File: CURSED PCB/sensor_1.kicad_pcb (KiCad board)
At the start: 4 copper layers, 40 x 40 mm, 68 parts, among them J1 Programming Header, J2 Micro_SD_Card, J3 2 Wire Block for laser, J4 2 Wire Block for PZT, J5 G125-MH104M4-04AD000P, U1 MIC94090YC6, U10 MCP2562, U11 TPS61046YFF, U12 AD5761BRUZ, U2 INA180, U3 STM32G431KBT6, U4 SPX3819M5-L-3-3, U5 MCP1754S-3302xCB, U6 OPA323, U7 MCP3562-E_ST, U8 LTC2066, Y1 24MHz crystal

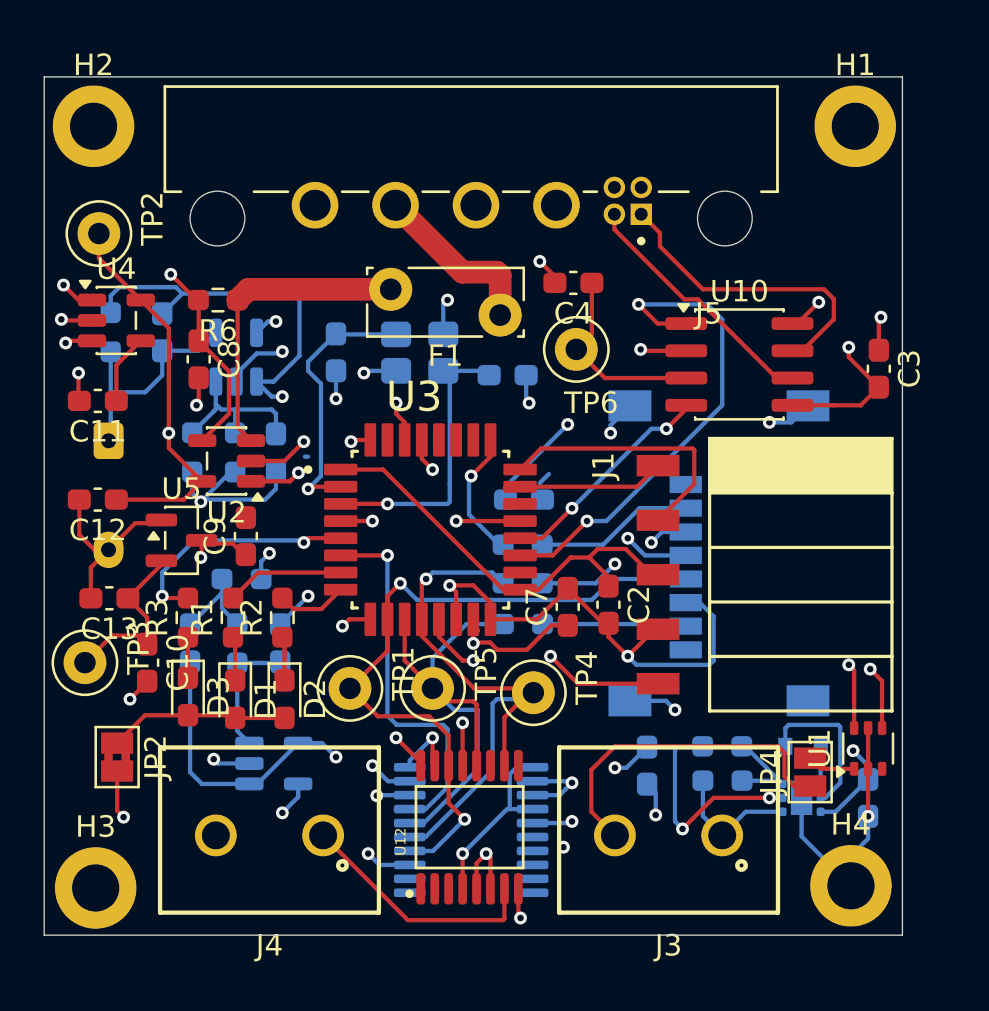
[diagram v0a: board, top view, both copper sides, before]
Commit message: redone pcb
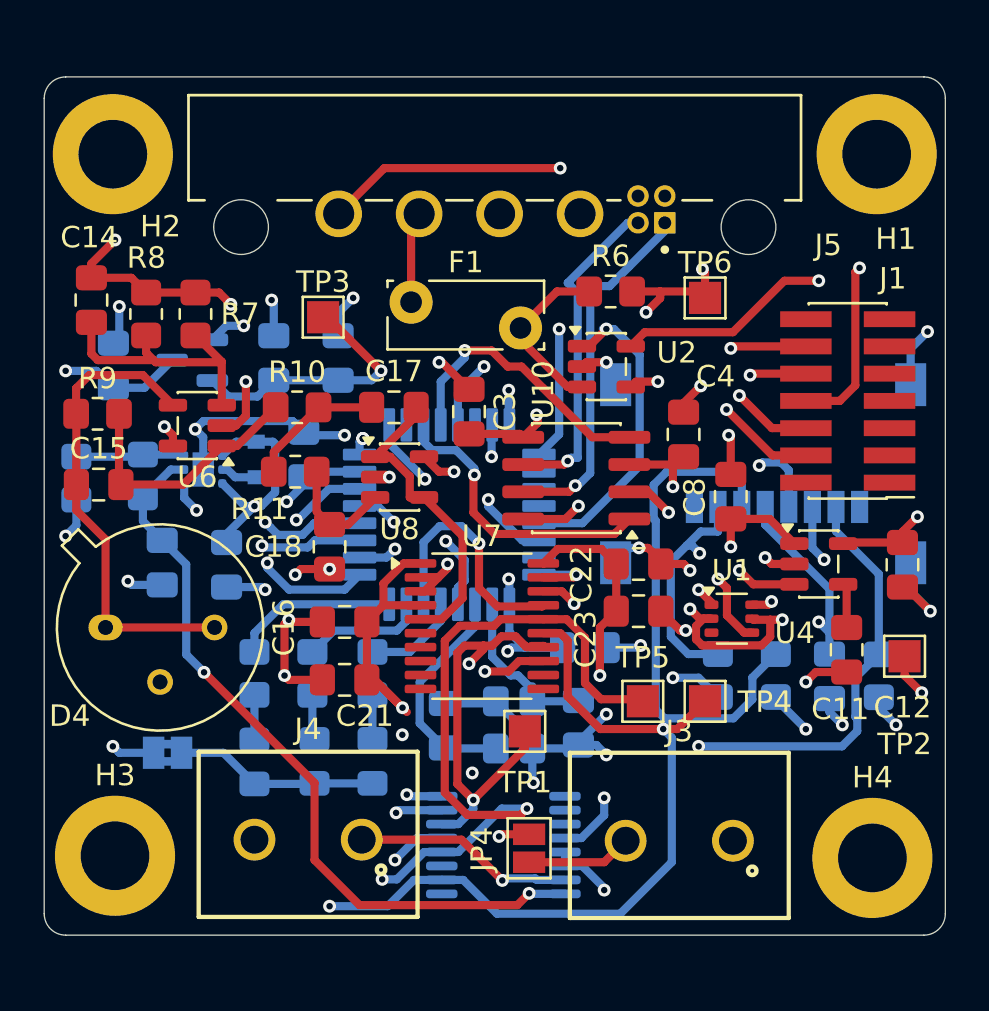
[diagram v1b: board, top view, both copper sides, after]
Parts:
- added C16: 0.1uF, Capacitor_SMD:C_0805_2012Metric_Pad1.18x1.45mm_HandSolder, F.Cu at (43.9, 55.4)
- added C21: 10uF, Capacitor_SMD:C_0805_2012Metric_Pad1.18x1.45mm_HandSolder, F.Cu at (43.9, 58.1)
- added C22: 0.1uF, Capacitor_SMD:C_0805_2012Metric_Pad1.18x1.45mm_HandSolder, F.Cu at (57.6, 52.7)
- added C23: 10uF, Capacitor_SMD:C_0805_2012Metric_Pad1.18x1.45mm_HandSolder, F.Cu at (57.6, 54.9)
- C1, C11, C12, C19, C20, C3, C4, C5, C6, C8: footprint Capacitor_SMD:C_0603_1608Metric_Pad1.08x0.95mm_HandSolder -> Capacitor_SMD:C_0805_2012Metric_Pad1.18x1.45mm_HandSolder
- C10, C13, C2, C7, C9: footprint Capacitor_SMD:C_0603_1608Metric_Pad1.08x0.95mm_HandSolder -> Capacitor_SMD:C_0805_2012Metric_Pad1.18x1.45mm_HandSolder; moved to B.Cu
- C14, C15, C17, C18: footprint Capacitor_SMD:C_0603_1608Metric_Pad1.08x0.95mm_HandSolder -> Capacitor_SMD:C_0805_2012Metric_Pad1.18x1.45mm_HandSolder; moved to F.Cu
- D1, D2, D3: footprint LED_SMD:LED_0603_1608Metric_Pad1.05x0.95mm_HandSolder -> LED_SMD:LED_0805_2012Metric_Pad1.15x1.40mm_HandSolder; moved to B.Cu
- D4: footprint OptoDevice:Osram_DIL2_4.3x4.65mm_P5.08mm -> Package_TO_SOT_THT:TO-5-3; moved to F.Cu
- H1, H2, H3, H4: footprint MountingHole:MountingHole_2.2mm_M2_DIN965_Pad -> MountingHole:MountingHole_3.2mm_M3_DIN965_Pad
- J1: value Programming Header -> Conn_02x07_Odd_Even; footprint canhw_footprints:PinSocket_5x2.54_SMD_90deg_952-3198-1-ND -> Connector_PinHeader_1.27mm:PinHeader_2x07_P1.27mm_Vertical_SMD
- JP2, U12, U3, U5: moved to B.Cu
- R1, R2, R3: footprint Resistor_SMD:R_0603_1608Metric_Pad0.98x0.95mm_HandSolder -> Resistor_SMD:R_0805_2012Metric_Pad1.20x1.40mm_HandSolder; moved to B.Cu
- R10, R11, R7, R8, R9: footprint Resistor_SMD:R_0603_1608Metric_Pad0.98x0.95mm_HandSolder -> Resistor_SMD:R_0805_2012Metric_Pad1.20x1.40mm_HandSolder; moved to F.Cu
- R12, R13, R14, R4, R5, R6: footprint Resistor_SMD:R_0603_1608Metric_Pad0.98x0.95mm_HandSolder -> Resistor_SMD:R_0805_2012Metric_Pad1.20x1.40mm_HandSolder
- TP1, TP2, TP3, TP4, TP5, TP6: footprint TestPoint:TestPoint_Loop_D2.50mm_Drill1.0mm -> TestPoint:TestPoint_Pad_1.5x1.5mm
- U6, U7, U8: moved to F.Cu
- moved TP2 42.4 mm to (70.0, 57.0), turned to 0 degrees
- moved C12 37.6 mm to (69.9, 52.7), turned to -90 degrees
- moved C11 36.8 mm to (67.3, 56.7), turned to -90 degrees
- moved U4 34.6 mm to (66.0, 52.7)
- moved R12 33.3 mm to (31.4, 48.7), turned to 90 degrees
- moved C19 31.8 mm to (38.4, 52.7)
- moved U11 31.8 mm to (37.3, 48.3)
- moved R13 29.8 mm to (34.5, 48.6), turned to -90 degrees
- moved L1 28.8 mm to (39.8, 47.8), turned to -90 degrees
- moved C8 25.6 mm to (61.9, 49.6), turned to 90 degrees
- moved C20 24.5 mm to (35.4, 52.6)
- moved C6 20.6 mm to (54.8, 60.1)
- moved TP3 19.6 mm to (42.9, 41.2), turned to 0 degrees
- moved C3 19.2 mm to (49.7, 45.6)
- moved R6 18.3 mm to (56.3, 40.0), turned to 0 degrees
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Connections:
- C10 pad 2: GND -> AGND
- C13 pad 2: GND -> AGND
- C14 pad 2: 5V -> +5V
- C15 pad 1: Net-(D4-K) -> Net-(D4-Cathode_2)
- C18 pad 2: GND -> AGND
- C19 pad 2: GND -> AGND
- C20 pad 2: GND -> AGND
- C3 pad 1: GND -> AGND
- C7 pad 2: GND -> AGND
- C9 pad 2: GND -> AGND
- D4 pad 1: Net-(D4-K) -> Net-(D4-Cathode_2)
- D4 pad 2: GND -> AGND
- H2 pad 1: GND -> AGND
- J1 pad 1: /PGC/ICSPDAT -> unconnected-(J1-Pin_1-Pad1)
- J1 pad 2: /PGD/ICSPCLK -> unconnected-(J1-Pin_2-Pad2)
- J1 pad 3: +3.3VD -> unconnected-(J1-Pin_3-Pad3)
- J1 pad 4: GND -> /PGC/ICSPDAT
- J1 pad 5: /MCLR -> unconnected-(J1-Pin_5-Pad5)
- J2 pad 2: Net-(J2-DAT3/CD) -> /CS2
- J2 pad 3: Net-(J2-CMD) -> /MOSI
- J2 pad 7: Net-(J2-DAT0) -> /MISO
- R12 pad 1: GND -> AGND
- R14 pad 1: /CS2 -> +3.3VD
- R14 pad 2: Net-(J2-DAT3/CD) -> /CS2
- R4 pad 1: /MOSI -> +3.3VD
- R4 pad 2: Net-(J2-CMD) -> /MOSI
- R5 pad 1: /MISO -> +3.3VD
- R5 pad 2: Net-(J2-DAT0) -> /MISO
- R7 pad 1: 5V -> +5V
- R8 pad 1: 5V -> +5V
- R9 pad 1: Net-(D4-K) -> Net-(D4-Cathode_2)
- U11 pad 1: GND -> AGND
- U11 pad 7: GND -> AGND
- U3 pad 14: GND -> AGND
- U5 pad 1: GND -> AGND
- U6 pad 2: GND -> AGND
- U6 pad 4: Net-(D4-K) -> Net-(D4-Cathode_2)
- U6 pad 5: 5V -> +5V
- U7 pad 2: GND -> AGND
- U7 pad 3: GND -> AGND
- U8 pad 2: GND -> AGND
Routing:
- net +5V: track 36.1 -> 112.6 mm, vias 7 -> 13
- net /MOSI: track 27.4 -> 90.1 mm, vias 1 -> 3
- net /MISO: track 23.8 -> 84.6 mm, vias 0 -> 4
- net +3.3VA: track 124.4 -> 76.4 mm, vias 4 -> 5
- net AGND: track 0.00 -> 43.3 mm, vias 0 -> 19
- net +3.3VD: track 109.4 -> 74.0 mm, vias 4 -> 14
- net /CS2: track 6.06 -> 32.1 mm, vias 1 -> 2
- net Net-(D4-Cathode_2): track 0.00 -> 22.1 mm
- net /SCLK: track 33.2 -> 54.9 mm, vias 3 -> 4
- net /Las_enable: track 42.4 -> 21.4 mm
- net 5V: track 19.5 -> 0.00 mm, vias 2 -> 0
- net Net-(JP4-B): track 2.26 -> 19.3 mm, vias 0 -> 2
- net /Amplifer/anti-aliasing filter/VIN: track 27.8 -> 12.0 mm, vias 2 -> 0
- net /MCLR: track 18.5 -> 34.2 mm
- net /CS_DAC: track 7.98 -> 21.3 mm
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- added copper zone on In1.Cu, net +3.3VD
- added copper zone on In2.Cu, net AGND
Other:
- board size 40 x 40 mm -> 42 x 40 mm

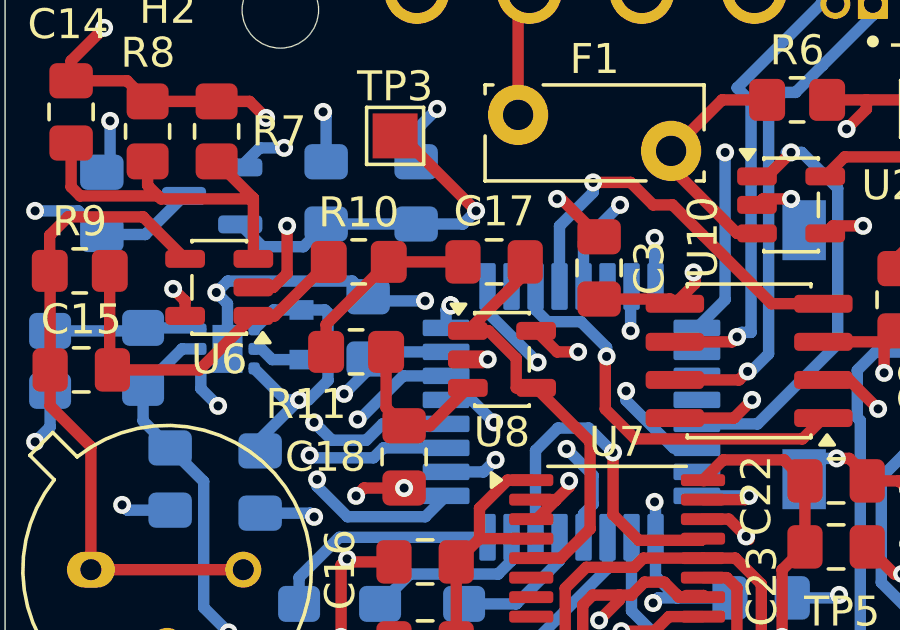
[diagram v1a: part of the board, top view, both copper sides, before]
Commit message: wires
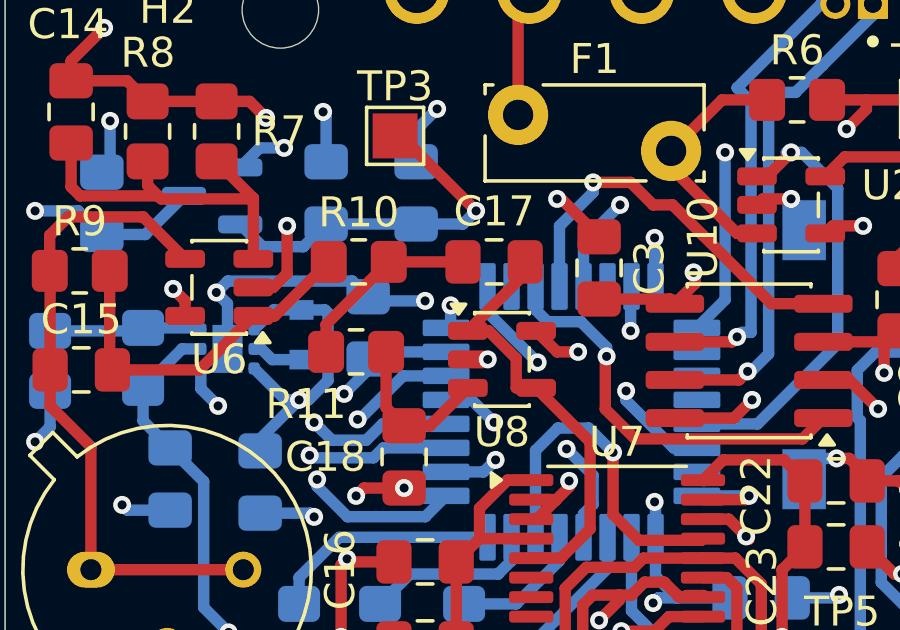
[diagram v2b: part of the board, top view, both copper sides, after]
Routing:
- net GND: vias 27 -> 26
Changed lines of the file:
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@@
+	)
+	(via
+		(at 44.75 46.85)
+		(size 0.6)
+		(drill 0.3)
+		(layers "F.Cu" "B.Cu")
+		(net 1)
 	)
 	(via
@@
 	)
 	(via
-		(at 44.75 46.85)
-		(size 0.6)
-		(drill 0.3)
-		(layers "F.Cu" "B.Cu")
-		(net 1)
-	)
-	(via
 		(at 71.07 41.87)
 		(size 0.6)
@@
 		(layers "F.Cu" "B.Cu")
 		(free yes)
-		(net 1)
-	)
-	(via
-		(at 44.75 46.85)
-		(size 0.6)
-		(drill 0.3)
-		(layers "F.Cu" "B.Cu")
 		(net 1)
 	)
@@
 	)
 	(segment
-		(start 44.6 47.6)
-		(end 44.6 47)
-		(width 0.381)
-		(layer "B.Cu")
-		(net 1)
-	)
-	(segment
 		(start 54.8 61.1375)
 		(end 55.6375 61.1375)
@@
 	)
 	(segment
-		(start 44.6 47)
-		(end 44.75 46.85)
+		(start 44.75 46.85)
+		(end 44.75 47.45)
 		(width 0.381)
 		(layer "B.Cu")
@@
 	)
 	(segment
+		(start 44.75 47.45)
+		(end 44.6 47.6)
+		(width 0.381)
+		(layer "B.Cu")
+		(net 1)
+	)
+	(segment
 		(start 56.5334 52.6166)
 		(end 56.5334 52.6431)
@@
 	)
 	(segment
-		(start 44.75 46.85)
-		(end 45.343055 46.85)
-		(width 0.381)
-		(layer "In2.Cu")
-		(net 1)
-	)
-	(segment
 		(start 46.9553 48.462245)
 		(end 46.9553 49.037755)
@@
 		(width 0.381)
 		(layer "In2.Cu")
+		(net 1)
+	)
+	(segment
+		(start 45.343055 46.85)
+		(end 44.75 46.85)
+		(width 0.381)
+		(layer "In2.Cu")
